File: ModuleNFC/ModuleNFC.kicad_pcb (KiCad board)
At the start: 2 copper layers, 49.5 x 38.8 mm, 42 parts, among them J1 Conn_01x10_Male, J2 Conn_01x04_Male, J3 Conn_01x08_Male, J4 Conn_Coaxial, Q1 2N7002DM, SW1 SW_DIP_x02, U1 PN5321A3HN_C1xx, Y1 27.12MHz

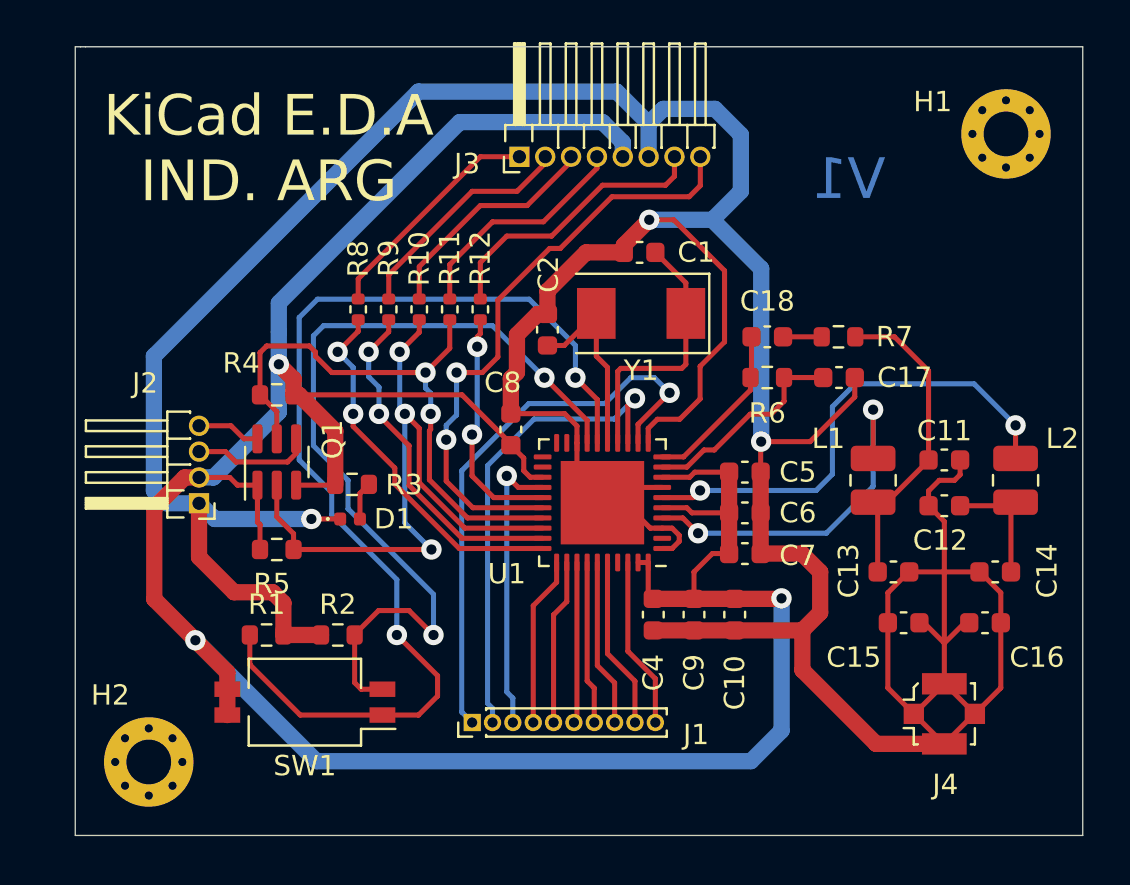
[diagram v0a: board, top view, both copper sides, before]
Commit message: All modification with correction
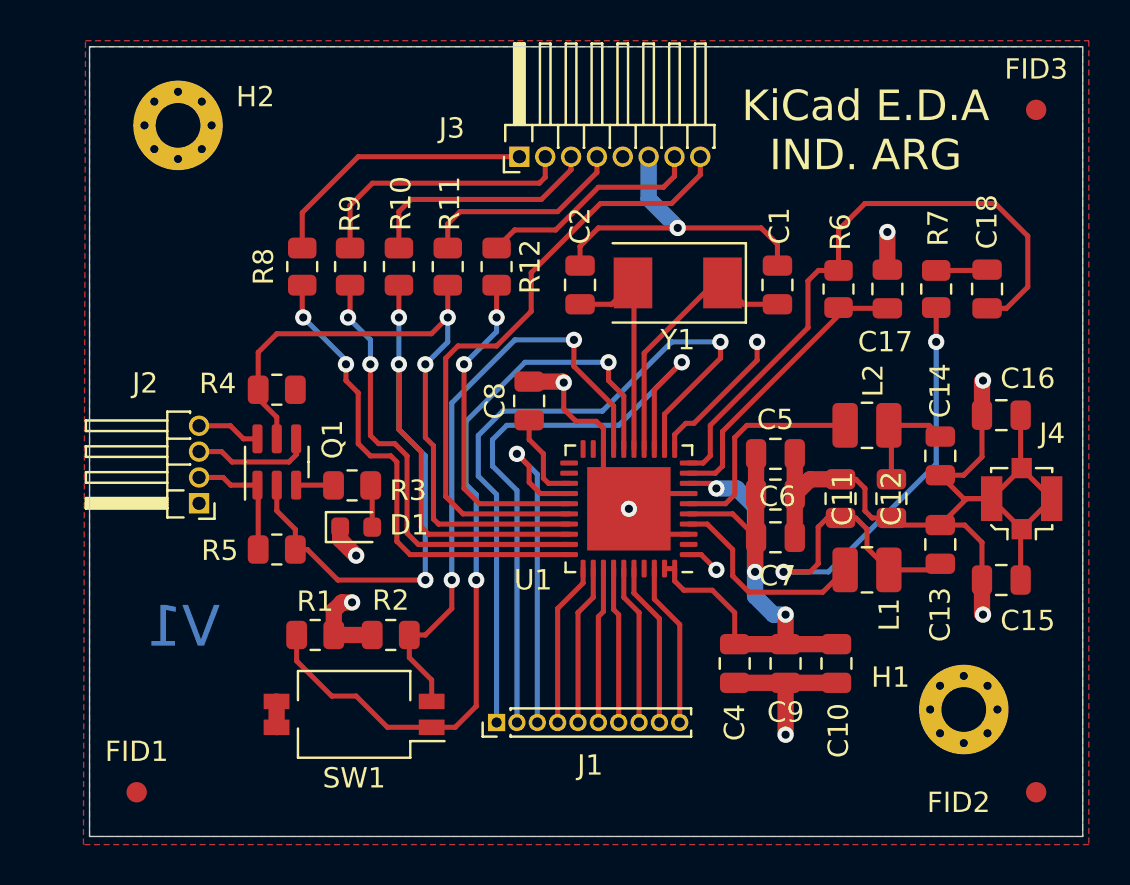
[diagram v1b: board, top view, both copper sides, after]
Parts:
- added FID1: Fiducial, Fiducial:Fiducial_1mm_Mask2mm, F.Cu at (128.0, 119.1)
- added FID2: Fiducial, Fiducial:Fiducial_1mm_Mask2mm, F.Cu at (172.2, 119.1)
- added FID3: Fiducial, Fiducial:Fiducial_1mm_Mask2mm, F.Cu at (172.2, 85.6)
- C1, C10, C11, C12, C13, C14, C15, C16, C17, C18, C2, C4, C5, C6, C7, C8, C9: footprint Capacitor_SMD:C_0603_1608Metric -> Capacitor_SMD:C_0805_2012Metric
- D1: footprint LED_SMD:LED_0402_1005Metric -> LED_SMD:LED_0603_1608Metric
- R1, R2, R3, R4, R5, R6, R7: footprint Resistor_SMD:R_0603_1608Metric -> Resistor_SMD:R_0805_2012Metric
- R10, R11, R12, R8, R9: footprint Resistor_SMD:R_0402_1005Metric -> Resistor_SMD:R_0805_2012Metric
- moved H2 31.3 mm to (130.0, 86.4)
- moved H1 28.4 mm to (168.7, 115.1)
- moved J4 11.2 mm to (171.5, 104.7), turned to 0 degrees
- moved C18 11.1 mm to (169.8, 94.4), turned to 270 degrees
- moved C16 10.2 mm to (170.5, 100.6)
- moved L2 7.78 mm to (163.9, 101.1), turned to 180 degrees
- moved C1 6.96 mm to (159.5, 94.2), turned to 90 degrees
- moved C14 6.31 mm to (167.5, 102.6), turned to 90 degrees
- moved R6 5.58 mm to (162.5, 94.4), turned to 270 degrees
- moved C10 5.55 mm to (162.4, 112.8)
- moved C11 5.44 mm to (162.6, 104.7), turned to 90 degrees
- moved R7 5.34 mm to (167.3, 94.4), turned to 270 degrees
- moved C15 5.24 mm to (170.5, 108.7), turned to 0 degrees
- moved C9 5.10 mm to (159.9, 112.8)
- moved C17 4.96 mm to (164.9, 94.4), turned to 90 degrees
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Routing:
- net GND: track 207.6 -> 102.2 mm, vias 3 -> 11
- net +3V3: track 137.8 -> 46.1 mm
- net Net-(C18-Pad2): track 8.33 -> 30.9 mm
- net Net-(R1-Pad1): track 53.6 -> 38.9 mm
- net Net-(C11-Pad1): track 15.8 -> 29.0 mm, vias 0 -> 2
- net Net-(L2-Pad2): track 24.1 -> 10.9 mm, vias 2 -> 0
- net Net-(R2-Pad1): track 42.6 -> 29.9 mm
- net /MOSI_SDA_TX: track 33.5 -> 41.6 mm
- net Net-(L1-Pad2): track 17.8 -> 10.3 mm, vias 2 -> 0
- net /AUX1: track 28.2 -> 34.7 mm
- net /AUX2: track 23.7 -> 30.1 mm
- net /SCK: track 18.2 -> 23.8 mm
- net /MISO: track 17.0 -> 22.1 mm
- net /NSS_SCL_RX: track 28.7 -> 33.5 mm
- net /IRQ: track 11.8 -> 16.1 mm
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- added copper zone on F.Cu, net +3V3
- added copper zone on B.Cu, net GND
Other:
- board size 49.5 x 38.8 mm -> 48.8 x 38.8 mm
- net class Default: clearance 0.2 -> 0.25
- rule trace_clearance: 0.2 -> 0.25
- board text added: "* Las restricciones para el ancho de las pistas son los utilizados por fabricantes de industria nacional. * Se utilizo las capacidades de fabricación nacional (Mayer). * La capacidad de Mayer planteada para este módulo fue 10 mils * La grilla utilizada para acomodar componente cómo primera aproximación fue 1mm * La grilla utilizada para routear las pistas fue 0.1mm * El módelo 3D de Q1 utilizado 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"
- board text removed: "* No se tiene restricciones sobre el tamaño de pistas. * Se utilizo las capacidades de fabricación nacional (Mayer). * La capacidad de Mayer planteada para este módulo fue 10 mils * La grilla utilizada para acomodar componente cómo primera aproximación fue 1mm * La grilla utilizada para routear las pistas fue 0.1mm"

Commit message: Export model 3D
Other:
- net class Default: clearance 0.25 -> 0.2
- rule trace_clearance: 0.25 -> 0.2
